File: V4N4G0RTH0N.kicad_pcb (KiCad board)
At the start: 2 copper layers, 122 parts, among them U1 ATmega32U4-A, Y1 16MHz

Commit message: I think I'm done??
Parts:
- removed F2: Polyfuse_Small, Fuse:Fuse_1206_3216Metric
- added U2: SRV05-4, Package_TO_SOT_SMD:SOT-23-6, B.Cu at (52.8, 32.3)
- moved R9 5.92 mm to (59.9, 25.1), turned to 180 degrees
- moved R8 5.30 mm to (45.7, 25.1), turned to 0 degrees
- moved R2 4.76 mm to (54.4, 38.9)
- moved R1 3.95 mm to (51.4, 38.9)
- moved C3 1.40 mm to (145.8, 122.2)
- moved USB1 1.27 mm to (52.8, 21.3)
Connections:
- R9 pad 1: Net-(R9-Pad1) -> GND
- R9 pad 2: GND -> Net-(R9-Pad2)
- USB1 pad 10: Net-(R9-Pad1) -> Net-(R9-Pad2)
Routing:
- net Net-(R2-Pad1): track 0.00 -> 225.8 mm, vias 0 -> 4
- net Net-(R1-Pad1): track 0.00 -> 223.1 mm, vias 0 -> 5
- net GND: track 81.4 -> 285.0 mm, vias 0 -> 4
- net (no net): track 0.00 -> 73.2 mm
- net D-: track 0.00 -> 21.4 mm, vias 0 -> 2
- net COL1: track 160.2 -> 179.6 mm
- net D+: track 0.00 -> 18.7 mm
- net VCC: track 0.00 -> 16.1 mm, vias 0 -> 4
- net COL8: track 84.7 -> 96.8 mm
- net COL4: track 121.3 -> 112.6 mm
- net Net-(R8-Pad2): track 0.00 -> 8.41 mm
- net Net-(R9-Pad2): track 0.00 -> 8.20 mm
- net +5V: track 63.5 -> 68.9 mm, vias 4 -> 6
- net COL5: track 118.7 -> 115.1 mm
- net Net-(C3-Pad1): track 2.26 -> 3.68 mm
- added copper zone on B.Cu, net GND
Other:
- board outline added: 247.7 x 102.9 mm

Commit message: Rev 1.0
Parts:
- added G***: LOGO, SILK:ORTHOVAN, F.Cu at (82.8, 83.2)
- moved R5 9.16 mm to (32.4, 34.5), turned to 180 degrees
- moved R6 9.04 mm to (32.4, 40.1), turned to 180 degrees
- moved R7 9.00 mm to (32.4, 46.1), turned to 180 degrees
- moved R8 4.73 mm to (45.2, 29.8)
- moved R9 4.73 mm to (59.4, 29.8)
- moved USB1 4.22 mm to (52.3, 25.5)
- moved R1 4.22 mm to (50.9, 43.1)
- moved R2 4.22 mm to (53.8, 43.1)
- moved U2 4.22 mm to (52.3, 36.4)
- moved D53 1.19 mm to (26.5, 42.8)
- moved D52 0.92 mm to (26.5, 37.2)
- moved D51 0.92 mm to (26.5, 31.7)
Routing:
- net (no net): track 73.2 -> 0.00 mm
- net GND: track 285.0 -> 275.7 mm, vias 4 -> 8
- net Net-(D53-Pad1): track 2.77 -> 10.9 mm
- net Net-(D51-Pad1): track 2.77 -> 10.9 mm
- net Net-(D52-Pad1): track 2.64 -> 9.92 mm
- net Net-(R2-Pad1): track 225.8 -> 221.4 mm
- net Net-(R1-Pad1): track 223.1 -> 219.2 mm
- net LED_2: track 178.2 -> 180.6 mm
- net LED_3: track 171.0 -> 173.3 mm
- net LED_1: track 184.4 -> 186.0 mm
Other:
- board size 247.7 x 102.9 mm -> 242.9 x 96.6 mm
- board text added: "V4N4G0RTH0N s8erdude"

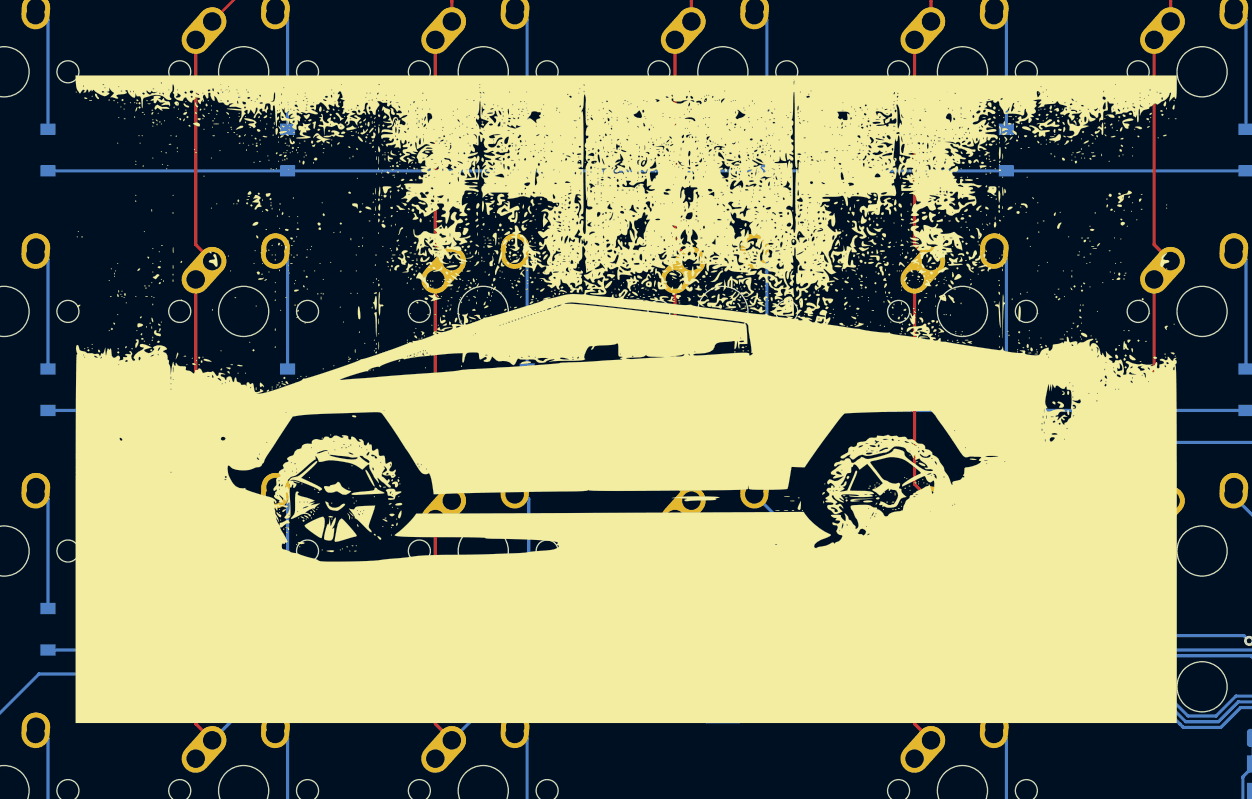
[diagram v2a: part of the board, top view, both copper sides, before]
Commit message: Add gerbers
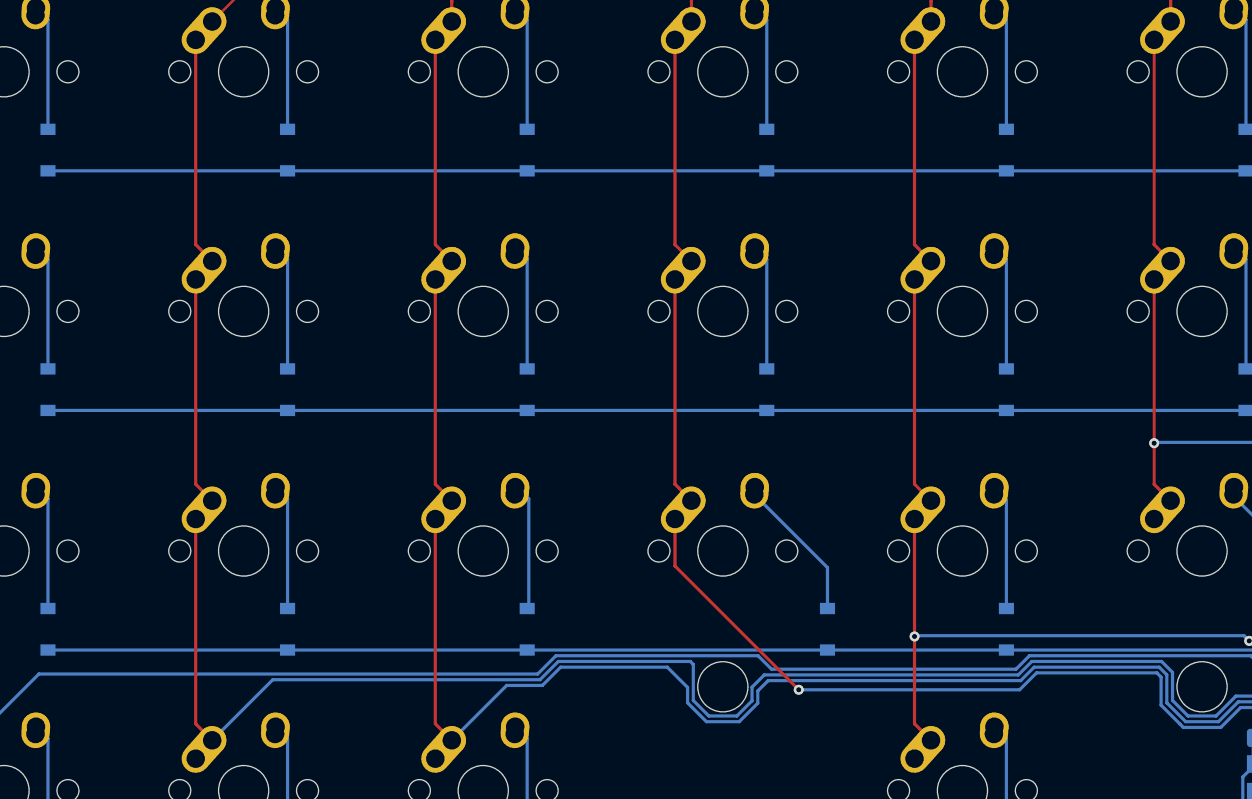
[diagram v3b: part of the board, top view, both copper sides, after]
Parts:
- removed G***: LOGO, SILK:ORTHOVAN
